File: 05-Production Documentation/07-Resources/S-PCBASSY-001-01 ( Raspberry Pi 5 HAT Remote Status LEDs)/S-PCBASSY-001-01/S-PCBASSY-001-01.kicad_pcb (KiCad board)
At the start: 2 copper layers, 65 x 56 mm, 43 parts, among them J1 GPIO, J2 43650-0428, Q1 BSS138, Q2 BSS138, Q3 BSS138, Q4 AO3401A, U1 CAT24C256

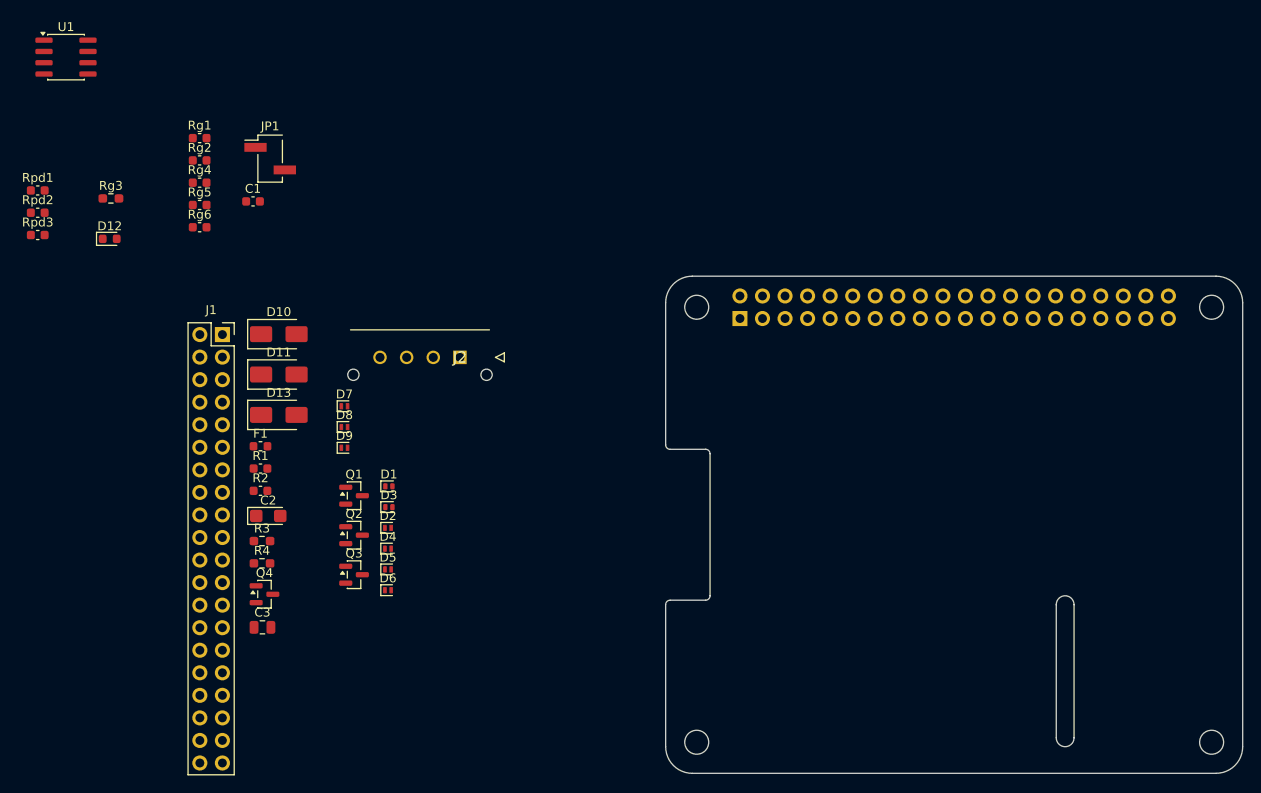
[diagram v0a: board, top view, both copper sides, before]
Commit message: Layout done
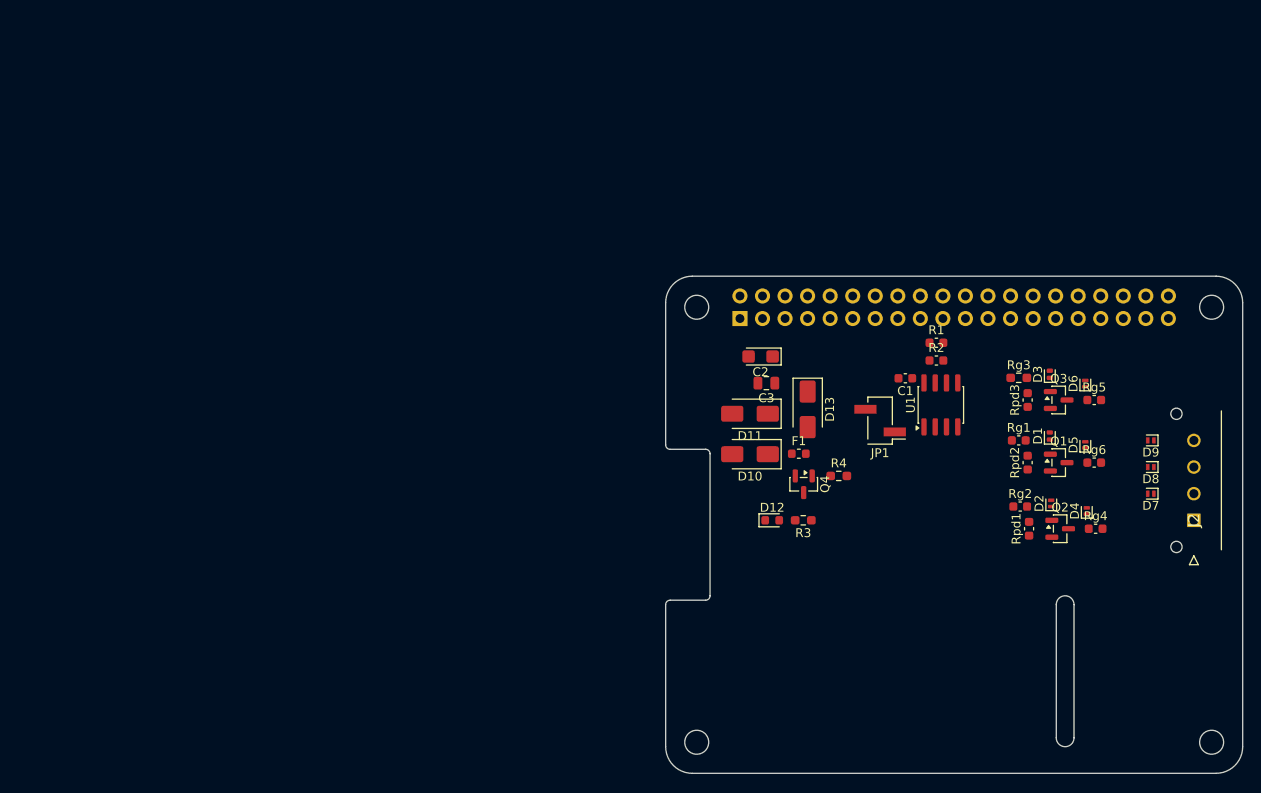
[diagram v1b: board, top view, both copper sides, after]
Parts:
- removed the J1 at (50.1, 50.6)
- moved Rpd1 118.0 mm to (140.9, 72.5), turned to 90 degrees
- moved Rpd2 115.0 mm to (140.8, 65.0), turned to 90 degrees
- moved Rpd3 113.0 mm to (140.8, 58.0), turned to 90 degrees
- moved Rg4 108.2 mm to (148.4, 72.5)
- moved U1 106.1 mm to (131.0, 58.5), turned to 90 degrees
- moved Rg3 104.2 mm to (139.8, 55.5)
- moved Rg6 104.2 mm to (148.3, 65.0)
- moved Rg5 103.1 mm to (148.3, 58.0)
- moved Rg2 100.3 mm to (139.9, 70.0)
- moved Rg1 98.4 mm to (139.8, 62.5)
- moved D7 91.4 mm to (154.7, 68.5), turned to 180 degrees
- moved D8 90.9 mm to (154.7, 65.5), turned to 180 degrees
- moved D9 90.8 mm to (154.7, 62.5), turned to 180 degrees
- moved J2 84.7 mm to (159.5, 71.5), turned to -90 degrees
- moved D6 81.9 mm to (147.3, 56.1), turned to 90 degrees
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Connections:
- C2 pad 1: Net-(D10-K) -> +5V
- C3 pad 1: Net-(D10-K) -> +5V
- D10 pad 1: Net-(D10-K) -> +5V
- D11 pad 1: Net-(D10-K) -> +5V
- F1 pad 1: Net-(D10-K) -> +5V
